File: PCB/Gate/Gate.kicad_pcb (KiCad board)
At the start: 2 copper layers, 124 x 124 mm, 236 parts, among them U1 QR

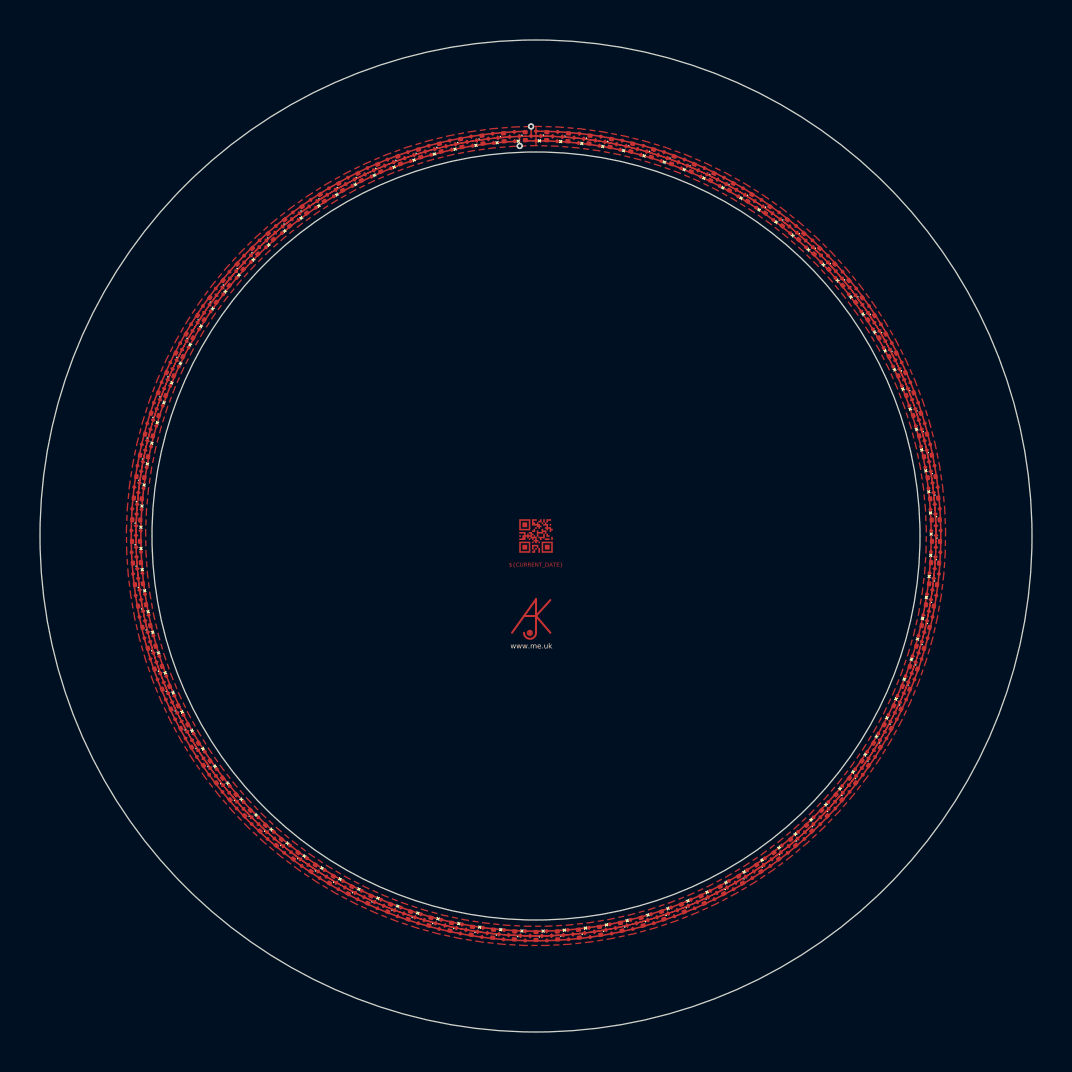
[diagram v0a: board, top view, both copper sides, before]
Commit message: Gate done
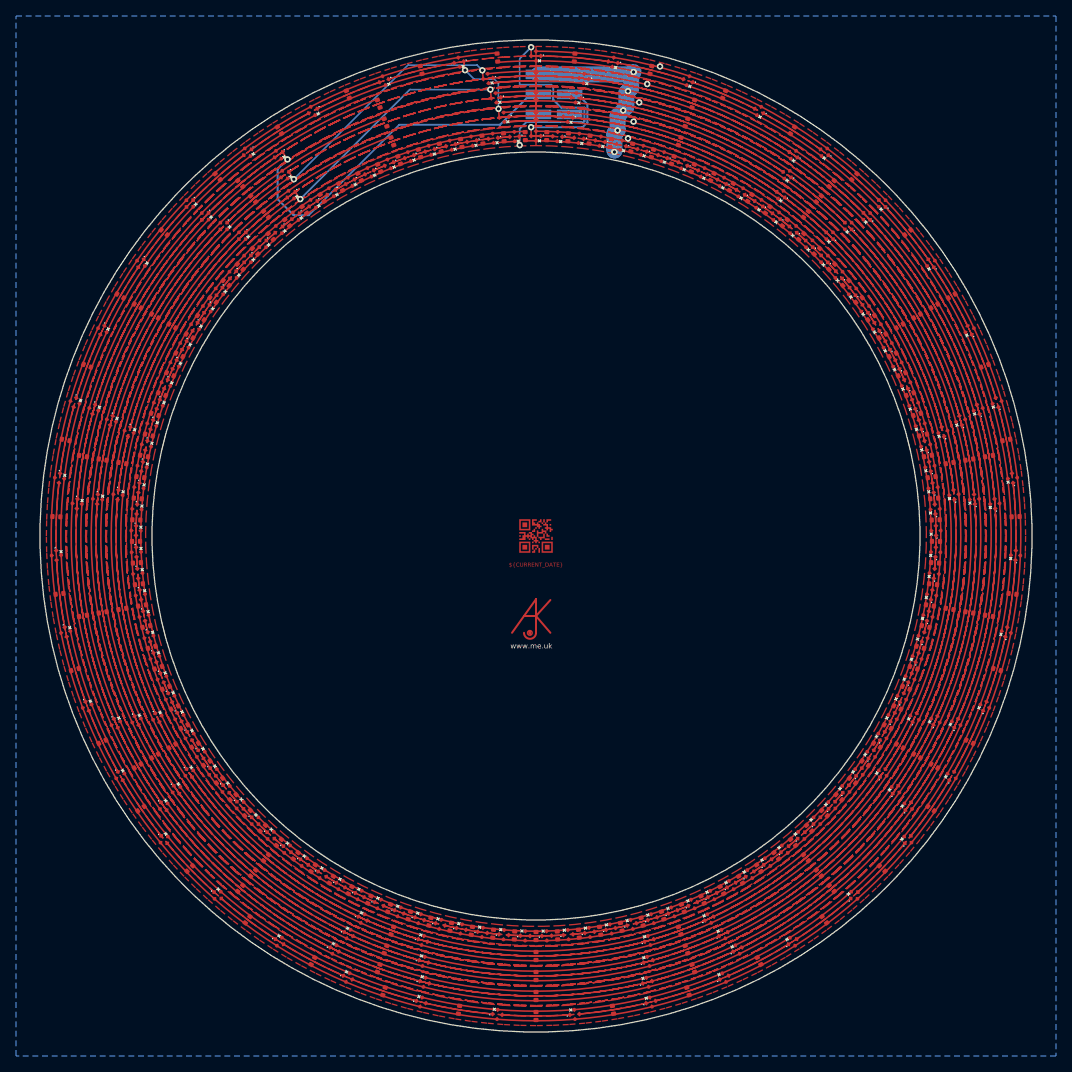
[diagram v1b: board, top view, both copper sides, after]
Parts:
- added C118: 330nF, RevK:C_0402, F.Cu at (104.8, 40.2)
- added C119: 330nF, RevK:C_0402, F.Cu at (114.4, 41.7)
- added C120: 330nF, RevK:C_0402, F.Cu at (123.5, 44.8)
- added C121: 330nF, RevK:C_0402, F.Cu at (132.1, 49.3)
- added C122: 330nF, RevK:C_0402, F.Cu at (139.8, 55.1)
- added C123: 330nF, RevK:C_0402, F.Cu at (146.5, 62.1)
- added C124: 330nF, RevK:C_0402, F.Cu at (152.0, 70.0)
- added C125: 330nF, RevK:C_0402, F.Cu at (156.1, 78.7)
- added C126: 330nF, RevK:C_0402, F.Cu at (158.8, 88.0)
- added C127: 330nF, RevK:C_0402, F.Cu at (160.0, 97.6)
- added C128: 330nF, RevK:C_0402, F.Cu at (159.6, 107.2)
- added C129: 330nF, RevK:C_0402, F.Cu at (157.6, 116.7)
- added C130: 330nF, RevK:C_0402, F.Cu at (154.2, 125.7)
- added C131: 330nF, RevK:C_0402, F.Cu at (149.4, 134.1)
- added C132: 330nF, RevK:C_0402, F.Cu at (143.3, 141.6)
- added C133: 330nF, RevK:C_0402, F.Cu at (136.0, 148.0)
- added C134: 330nF, RevK:C_0402, F.Cu at (127.9, 153.1)
- added C135: 330nF, RevK:C_0402, F.Cu at (119.0, 156.9)
- added C136: 330nF, RevK:C_0402, F.Cu at (109.6, 159.2)
- added C137: 330nF, RevK:C_0402, F.Cu at (100.0, 160.0)
- added C138: 330nF, RevK:C_0402, F.Cu at (90.4, 159.2)
- added C139: 330nF, RevK:C_0402, F.Cu at (81.0, 156.9)
- added C140: 330nF, RevK:C_0402, F.Cu at (72.1, 153.1)
- added C141: 330nF, RevK:C_0402, F.Cu at (64.0, 148.0)
- added C142: 330nF, RevK:C_0402, F.Cu at (56.7, 141.6)
- added C143: 330nF, RevK:C_0402, F.Cu at (50.6, 134.1)
- added C144: 330nF, RevK:C_0402, F.Cu at (45.8, 125.7)
- added C145: 330nF, RevK:C_0402, F.Cu at (42.4, 116.7)
- added C146: 330nF, RevK:C_0402, F.Cu at (40.4, 107.2)
- added C147: 330nF, RevK:C_0402, F.Cu at (40.0, 97.6)
- added C148: 330nF, RevK:C_0402, F.Cu at (41.2, 88.0)
- added C149: 330nF, RevK:C_0402, F.Cu at (43.9, 78.7)
- added C150: 330nF, RevK:C_0402, F.Cu at (48.0, 70.0)
- added C151: 330nF, RevK:C_0402, F.Cu at (53.5, 62.1)
- added C152: 330nF, RevK:C_0402, F.Cu at (60.2, 55.1)
- added C153: 330nF, RevK:C_0402, F.Cu at (67.9, 49.3)
- added C154: 330nF, RevK:C_0402, F.Cu at (76.5, 44.8)
- added C155: 330nF, RevK:C_0402, F.Cu at (85.6, 41.7)
- added C156: 330nF, RevK:C_0402, F.Cu at (95.2, 40.2)
- added C157: 330nF, RevK:C_0402, F.Cu at (100.0, 47.5)
- added C158: 330nF, RevK:C_0402, F.Cu at (118.0, 50.7)
- added C159: 330nF, RevK:C_0402, F.Cu at (133.7, 59.8)
- added C160: 330nF, RevK:C_0402, F.Cu at (145.5, 73.8)
- added C161: 330nF, RevK:C_0402, F.Cu at (151.7, 90.9)
- added C162: 330nF, RevK:C_0402, F.Cu at (151.7, 109.1)
- added C163: 330nF, RevK:C_0402, F.Cu at (145.5, 126.2)
- added C164: 330nF, RevK:C_0402, F.Cu at (133.7, 140.2)
- added C165: 330nF, RevK:C_0402, F.Cu at (118.0, 149.3)
- added C166: 330nF, RevK:C_0402, F.Cu at (100.0, 152.5)
- added C167: 330nF, RevK:C_0402, F.Cu at (82.0, 149.3)
- added C168: 330nF, RevK:C_0402, F.Cu at (66.3, 140.2)
- added C169: 330nF, RevK:C_0402, F.Cu at (54.5, 126.2)
- added C170: 330nF, RevK:C_0402, F.Cu at (48.3, 109.1)
- added C171: 330nF, RevK:C_0402, F.Cu at (48.3, 90.9)
- added C172: 330nF, RevK:C_0402, F.Cu at (54.5, 73.8)
- added C173: 330nF, RevK:C_0402, F.Cu at (66.3, 59.8)
- added C174: 330nF, RevK:C_0402, F.Cu at (82.0, 50.7)
- added C175: 330nF, RevK:C_0402, F.Cu at (100.0, 45.0)
- added C176: 330nF, RevK:C_0402, F.Cu at (118.8, 48.3)
- added C177: 330nF, RevK:C_0402, F.Cu at (135.4, 57.9)
- added C178: 330nF, RevK:C_0402, F.Cu at (147.6, 72.5)
- added C179: 330nF, RevK:C_0402, F.Cu at (154.2, 90.4)
- added C180: 330nF, RevK:C_0402, F.Cu at (154.2, 109.6)
- added C181: 330nF, RevK:C_0402, F.Cu at (147.6, 127.5)
- added C182: 330nF, RevK:C_0402, F.Cu at (135.4, 142.1)
- added C183: 330nF, RevK:C_0402, F.Cu at (118.8, 151.7)
- added C184: 330nF, RevK:C_0402, F.Cu at (100.0, 155.0)
- added C185: 330nF, RevK:C_0402, F.Cu at (81.2, 151.7)
- added C186: 330nF, RevK:C_0402, F.Cu at (64.6, 142.1)
- added C187: 330nF, RevK:C_0402, F.Cu at (52.4, 127.5)
- added C188: 330nF, RevK:C_0402, F.Cu at (45.8, 109.6)
- added C189: 330nF, RevK:C_0402, F.Cu at (45.8, 90.4)
- added C190: 330nF, RevK:C_0402, F.Cu at (52.4, 72.5)
- added C191: 330nF, RevK:C_0402, F.Cu at (64.6, 57.9)
- added C192: 330nF, RevK:C_0402, F.Cu at (81.2, 48.3)
- added C193: 330nF, RevK:C_0402, F.Cu at (100.0, 42.5)
- added C194: 330nF, RevK:C_0402, F.Cu at (119.7, 46.0)
- added C195: 330nF, RevK:C_0402, F.Cu at (137.0, 56.0)
- added C196: 330nF, RevK:C_0402, F.Cu at (149.8, 71.2)
- added C197: 330nF, RevK:C_0402, F.Cu at (156.6, 90.0)
- added C198: 330nF, RevK:C_0402, F.Cu at (156.6, 110.0)
- added C199: 330nF, RevK:C_0402, F.Cu at (149.8, 128.8)
- added C200: 330nF, RevK:C_0402, F.Cu at (137.0, 144.0)
- added C201: 330nF, RevK:C_0402, F.Cu at (119.7, 154.0)
- added C202: 330nF, RevK:C_0402, F.Cu at (100.0, 157.5)
- added C203: 330nF, RevK:C_0402, F.Cu at (80.3, 154.0)
- added C204: 330nF, RevK:C_0402, F.Cu at (63.0, 144.0)
- added C205: 330nF, RevK:C_0402, F.Cu at (50.2, 128.8)
- added C206: 330nF, RevK:C_0402, F.Cu at (43.4, 110.0)
- added C207: 330nF, RevK:C_0402, F.Cu at (43.4, 90.0)
- added C208: 330nF, RevK:C_0402, F.Cu at (50.2, 71.2)
- added C209: 330nF, RevK:C_0402, F.Cu at (63.0, 56.0)
- added C210: 330nF, RevK:C_0402, F.Cu at (80.3, 46.0)
- added D118: XL-1010RGBC-WS2812B, RevK:SMD1010, F.Cu at (100.0, 40.0)
- added D119: XL-1010RGBC-WS2812B, RevK:SMD1010, F.Cu at (109.6, 40.8)
- added D120: XL-1010RGBC-WS2812B, RevK:SMD1010, F.Cu at (119.0, 43.1)
- added D121: XL-1010RGBC-WS2812B, RevK:SMD1010, F.Cu at (127.9, 46.9)
- added D122: XL-1010RGBC-WS2812B, RevK:SMD1010, F.Cu at (136.0, 52.0)
- added D123: XL-1010RGBC-WS2812B, RevK:SMD1010, F.Cu at (143.3, 58.4)
- added D124: XL-1010RGBC-WS2812B, RevK:SMD1010, F.Cu at (149.4, 65.9)
- added D125: XL-1010RGBC-WS2812B, RevK:SMD1010, F.Cu at (154.2, 74.3)
- added D126: XL-1010RGBC-WS2812B, RevK:SMD1010, F.Cu at (157.6, 83.3)
- added D127: XL-1010RGBC-WS2812B, RevK:SMD1010, F.Cu at (159.6, 92.8)
- added D128: XL-1010RGBC-WS2812B, RevK:SMD1010, F.Cu at (160.0, 102.4)
- added D129: XL-1010RGBC-WS2812B, RevK:SMD1010, F.Cu at (158.8, 112.0)
- added D130: XL-1010RGBC-WS2812B, RevK:SMD1010, F.Cu at (156.1, 121.3)
- added D131: XL-1010RGBC-WS2812B, RevK:SMD1010, F.Cu at (152.0, 130.0)
- added D132: XL-1010RGBC-WS2812B, RevK:SMD1010, F.Cu at (146.5, 137.9)
- added D133: XL-1010RGBC-WS2812B, RevK:SMD1010, F.Cu at (139.8, 144.9)
- added D134: XL-1010RGBC-WS2812B, RevK:SMD1010, F.Cu at (132.1, 150.7)
- added D135: XL-1010RGBC-WS2812B, RevK:SMD1010, F.Cu at (123.5, 155.2)
- added D136: XL-1010RGBC-WS2812B, RevK:SMD1010, F.Cu at (114.4, 158.3)
- added D137: XL-1010RGBC-WS2812B, RevK:SMD1010, F.Cu at (104.8, 159.8)
- added D138: XL-1010RGBC-WS2812B, RevK:SMD1010, F.Cu at (95.2, 159.8)
- added D139: XL-1010RGBC-WS2812B, RevK:SMD1010, F.Cu at (85.6, 158.3)
- added D140: XL-1010RGBC-WS2812B, RevK:SMD1010, F.Cu at (76.5, 155.2)
- added D141: XL-1010RGBC-WS2812B, RevK:SMD1010, F.Cu at (67.9, 150.7)
- added D142: XL-1010RGBC-WS2812B, RevK:SMD1010, F.Cu at (60.2, 144.9)
- added D143: XL-1010RGBC-WS2812B, RevK:SMD1010, F.Cu at (53.5, 137.9)
- added D144: XL-1010RGBC-WS2812B, RevK:SMD1010, F.Cu at (48.0, 130.0)
- added D145: XL-1010RGBC-WS2812B, RevK:SMD1010, F.Cu at (43.9, 121.3)
- added D146: XL-1010RGBC-WS2812B, RevK:SMD1010, F.Cu at (41.2, 112.0)
- added D147: XL-1010RGBC-WS2812B, RevK:SMD1010, F.Cu at (40.0, 102.4)
- added D148: XL-1010RGBC-WS2812B, RevK:SMD1010, F.Cu at (40.4, 92.8)
- added D149: XL-1010RGBC-WS2812B, RevK:SMD1010, F.Cu at (42.4, 83.3)
- added D150: XL-1010RGBC-WS2812B, RevK:SMD1010, F.Cu at (45.8, 74.3)
- added D151: XL-1010RGBC-WS2812B, RevK:SMD1010, F.Cu at (50.6, 65.9)
- added D152: XL-1010RGBC-WS2812B, RevK:SMD1010, F.Cu at (56.7, 58.4)
- added D153: XL-1010RGBC-WS2812B, RevK:SMD1010, F.Cu at (64.0, 52.0)
- added D154: XL-1010RGBC-WS2812B, RevK:SMD1010, F.Cu at (72.1, 46.9)
- added D155: XL-1010RGBC-WS2812B, RevK:SMD1010, F.Cu at (81.0, 43.1)
- added D156: XL-1010RGBC-WS2812B, RevK:SMD1010, F.Cu at (90.4, 40.8)
- added D157: XL-1010RGBC-WS2812B, RevK:SMD1010, F.Cu at (96.0, 47.7)
- added D158: XL-1010RGBC-WS2812B, RevK:SMD1010, F.Cu at (104.0, 47.7)
- added D159: XL-1010RGBC-WS2812B, RevK:SMD1010, F.Cu at (130.6, 57.3)
- added D160: XL-1010RGBC-WS2812B, RevK:SMD1010, F.Cu at (136.7, 62.5)
- added D161: XL-1010RGBC-WS2812B, RevK:SMD1010, F.Cu at (150.9, 87.0)
- added D162: XL-1010RGBC-WS2812B, RevK:SMD1010, F.Cu at (152.2, 94.8)
- added D163: XL-1010RGBC-WS2812B, RevK:SMD1010, F.Cu at (147.3, 122.7)
- added D164: XL-1010RGBC-WS2812B, RevK:SMD1010, F.Cu at (143.3, 129.6)
- added D165: XL-1010RGBC-WS2812B, RevK:SMD1010, F.Cu at (121.7, 147.8)
- added D166: XL-1010RGBC-WS2812B, RevK:SMD1010, F.Cu at (114.1, 150.6)
- added D167: XL-1010RGBC-WS2812B, RevK:SMD1010, F.Cu at (85.9, 150.6)
- added D168: XL-1010RGBC-WS2812B, RevK:SMD1010, F.Cu at (78.3, 147.8)
- added D169: XL-1010RGBC-WS2812B, RevK:SMD1010, F.Cu at (56.7, 129.6)
- added D170: XL-1010RGBC-WS2812B, RevK:SMD1010, F.Cu at (52.7, 122.7)
- added D171: XL-1010RGBC-WS2812B, RevK:SMD1010, F.Cu at (47.8, 94.8)
- added D172: XL-1010RGBC-WS2812B, RevK:SMD1010, F.Cu at (49.1, 87.0)
- added D173: XL-1010RGBC-WS2812B, RevK:SMD1010, F.Cu at (63.3, 62.5)
- added D174: XL-1010RGBC-WS2812B, RevK:SMD1010, F.Cu at (69.4, 57.3)
- added D175: XL-1010RGBC-WS2812B, RevK:SMD1010, F.Cu at (95.0, 45.2)
- added D176: XL-1010RGBC-WS2812B, RevK:SMD1010, F.Cu at (105.0, 45.2)
- added D177: XL-1010RGBC-WS2812B, RevK:SMD1010, F.Cu at (131.4, 54.8)
- added D178: XL-1010RGBC-WS2812B, RevK:SMD1010, F.Cu at (139.0, 61.3)
- added D179: XL-1010RGBC-WS2812B, RevK:SMD1010, F.Cu at (153.1, 85.6)
- added D180: XL-1010RGBC-WS2812B, RevK:SMD1010, F.Cu at (154.8, 95.4)
- added D181: XL-1010RGBC-WS2812B, RevK:SMD1010, F.Cu at (149.9, 123.1)
- added D182: XL-1010RGBC-WS2812B, RevK:SMD1010, F.Cu at (144.9, 131.7)
- added D183: XL-1010RGBC-WS2812B, RevK:SMD1010, F.Cu at (123.4, 149.8)
- added D184: XL-1010RGBC-WS2812B, RevK:SMD1010, F.Cu at (114.0, 153.2)
- added D185: XL-1010RGBC-WS2812B, RevK:SMD1010, F.Cu at (86.0, 153.2)
- added D186: XL-1010RGBC-WS2812B, RevK:SMD1010, F.Cu at (76.6, 149.8)
- added D187: XL-1010RGBC-WS2812B, RevK:SMD1010, F.Cu at (55.1, 131.7)
- added D188: XL-1010RGBC-WS2812B, RevK:SMD1010, F.Cu at (50.1, 123.1)
- added D189: XL-1010RGBC-WS2812B, RevK:SMD1010, F.Cu at (45.2, 95.4)
- added D190: XL-1010RGBC-WS2812B, RevK:SMD1010, F.Cu at (46.9, 85.6)
- added D191: XL-1010RGBC-WS2812B, RevK:SMD1010, F.Cu at (61.0, 61.3)
- added D192: XL-1010RGBC-WS2812B, RevK:SMD1010, F.Cu at (68.6, 54.8)
- added D193: XL-1010RGBC-WS2812B, RevK:SMD1010, F.Cu at (94.0, 42.8)
- added D194: XL-1010RGBC-WS2812B, RevK:SMD1010, F.Cu at (106.0, 42.8)
- added D195: XL-1010RGBC-WS2812B, RevK:SMD1010, F.Cu at (132.2, 52.3)
- added D196: XL-1010RGBC-WS2812B, RevK:SMD1010, F.Cu at (141.3, 60.0)
- added D197: XL-1010RGBC-WS2812B, RevK:SMD1010, F.Cu at (155.3, 84.2)
- added D198: XL-1010RGBC-WS2812B, RevK:SMD1010, F.Cu at (157.4, 96.0)
- added D199: XL-1010RGBC-WS2812B, RevK:SMD1010, F.Cu at (152.5, 123.4)
- added D200: XL-1010RGBC-WS2812B, RevK:SMD1010, F.Cu at (146.5, 133.8)
- added D201: XL-1010RGBC-WS2812B, RevK:SMD1010, F.Cu at (125.2, 151.7)
- added D202: XL-1010RGBC-WS2812B, RevK:SMD1010, F.Cu at (113.9, 155.8)
- added D203: XL-1010RGBC-WS2812B, RevK:SMD1010, F.Cu at (86.1, 155.8)
- added D204: XL-1010RGBC-WS2812B, RevK:SMD1010, F.Cu at (74.8, 151.7)
- added D205: XL-1010RGBC-WS2812B, RevK:SMD1010, F.Cu at (53.5, 133.8)
- added D206: XL-1010RGBC-WS2812B, RevK:SMD1010, F.Cu at (47.5, 123.4)
- added D207: XL-1010RGBC-WS2812B, RevK:SMD1010, F.Cu at (42.6, 96.0)
- added D208: XL-1010RGBC-WS2812B, RevK:SMD1010, F.Cu at (44.7, 84.2)
- added D209: XL-1010RGBC-WS2812B, RevK:SMD1010, F.Cu at (58.7, 60.0)
- added D210: XL-1010RGBC-WS2812B, RevK:SMD1010, F.Cu at (67.8, 52.3)
- added J1: Conn_01x03, RevK:3-PADS, B.Cu at (104.2, 44.8)
- added J2: Conn_01x03, RevK:3-PADS, B.Cu at (100.3, 44.8)
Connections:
- D1 pad 4: unconnected-(D1-I-Pad4) -> Net-(D1-I)
- D117 pad 1: unconnected-(D117-O-Pad1) -> Net-(D117-O)
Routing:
- net GND: track 0.00 -> 1695.3 mm, vias 0 -> 5
- net VCC: track 0.00 -> 1661.4 mm, vias 0 -> 5
- net (no net): track 800.0 -> 0.00 mm, vias 2 -> 0
- net Net-(D210-O): track 0.00 -> 46.3 mm, vias 0 -> 1
- net Net-(D192-O): track 0.00 -> 31.9 mm, vias 0 -> 2
- net Net-(D174-O): track 0.00 -> 31.6 mm, vias 0 -> 2
- net Net-(D117-O): track 0.00 -> 30.0 mm, vias 0 -> 2
- net Net-(D172-O): track 0.00 -> 27.4 mm
- net Net-(D160-O): track 0.00 -> 27.4 mm
- net Net-(D166-O): track 0.00 -> 27.4 mm
- net Net-(D170-O): track 0.00 -> 27.4 mm
- net Net-(D162-O): track 0.00 -> 27.4 mm
- net Net-(D164-O): track 0.00 -> 27.4 mm
- net Net-(D168-O): track 0.00 -> 27.4 mm
- net Net-(D158-O): track 0.00 -> 27.4 mm
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- added copper zone on B.Cu, net GND
